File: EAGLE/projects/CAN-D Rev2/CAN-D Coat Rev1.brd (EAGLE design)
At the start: 55.3 x 89.2 mm, 10 parts, among them P1 LCW-106-XX-X-S, P2 LCW-106-XX-X-S, SW1 SCHURTER-LSH-1301.9314, SW2 SCHURTER-LSH-1301.9314, SW3 SCHURTER-LSH-1301.9314

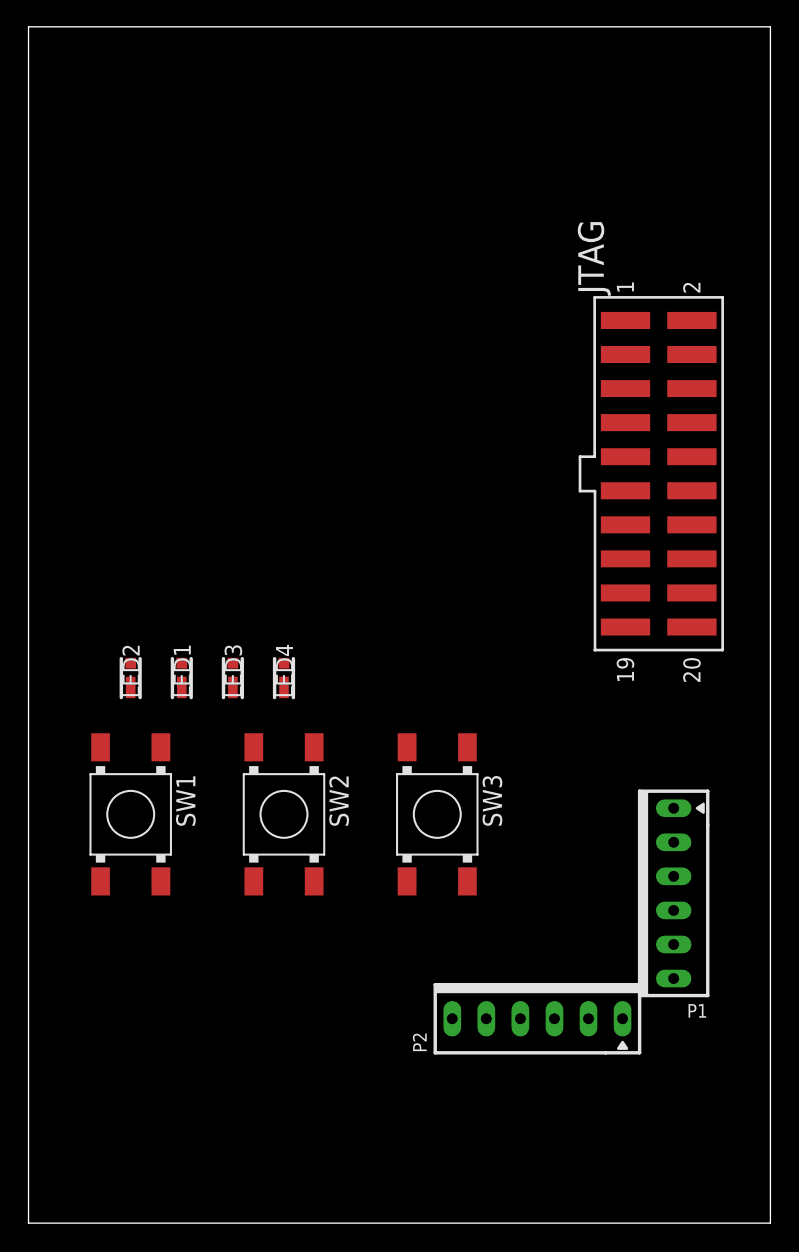
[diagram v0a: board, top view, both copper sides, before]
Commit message: Clean up EAGLE files
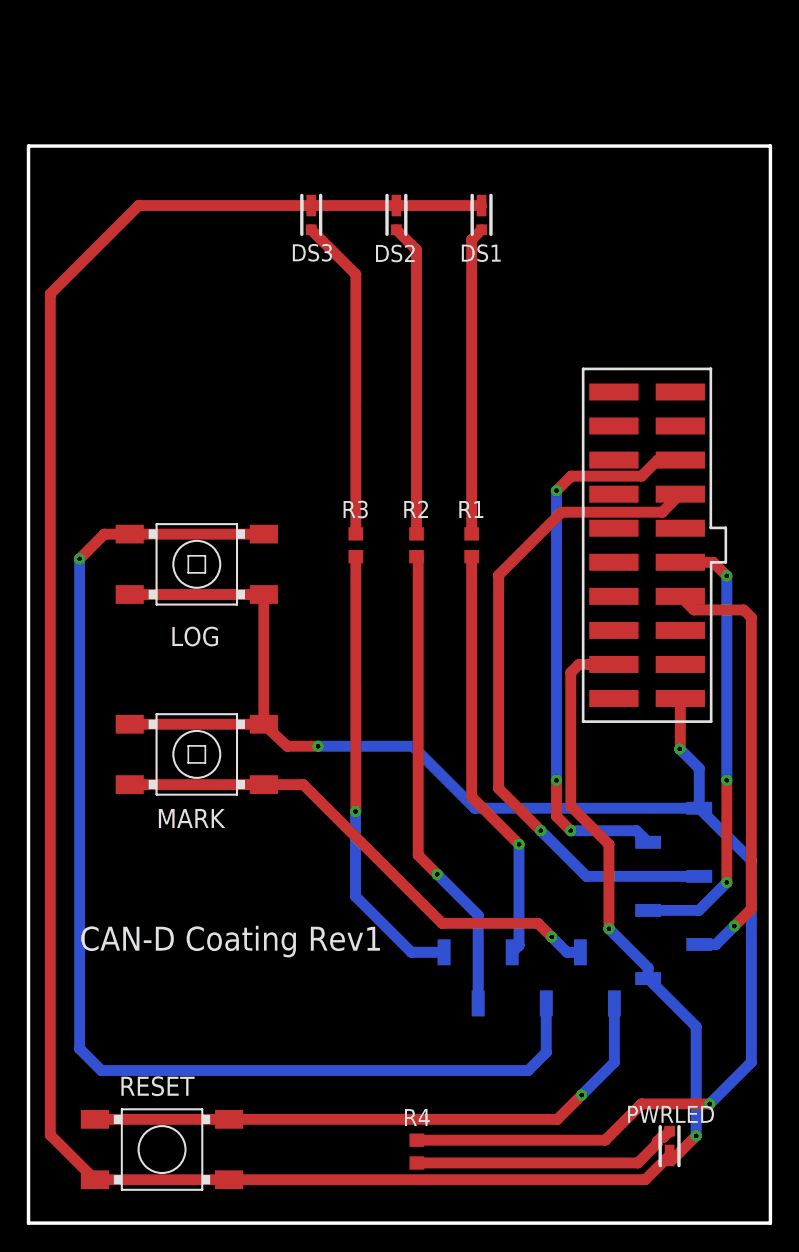
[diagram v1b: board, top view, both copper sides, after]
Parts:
- removed LED1, LED2, LED3, LED4: L130-6580001400001, L130-6580001400001:L130-6580001400001
- removed P1, P2: LCW-106-XX-X-S, con-samtec:LCW-106-XX-X-S
- removed SW1, SW2, SW3: SCHURTER-LSH-1301.9314, schurter_switches_LSH_SMS:LSH
- added DS1, DS2, DS3, PWRLED: LED, CAN-D:L130-6580001400001
- added J1, J2: RECEPTACLE, CAN-D:SSM-106-L-SV-K-TR
- added LOG, MARK: BUTTONSPLUNGER, CAN-D:TL3301SPF260QG
- added R1, R2, R4: 550, CAN-D:R0603
- added R3: 550, rcl:R0603
- added RESET: BUTTONS, CAN-D:1301.9314
- JTAG: value SAMTEC-TSM-110-01-X-DVJ -> JTAG-HEADERJ; device SAMTEC-TSM-110-01-X-DV:SAMTEC-TSM-110-01-X-DV -> CAN-D:TSM-110-02-L-DV-A-P-TR
- moved JTAG 5.40 mm to (46.1, 50.5), turned to 90 degrees
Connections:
- removed net N$1: P1.1
- removed net N$11: P2.5
- removed net N$12: P2.6
- removed net N$2: P1.2
- removed net N$3: P1.3
- removed net N$4: P1.4
- removed net N$5: P1.5
- removed net N$6: P1.6
- new net GND: DS1.2, DS2.2, DS3.2, J1.6, JTAG.4, PWRLED.2, RESET.NO1, RESET.NO2
- new net LED1: J2.3, R1.1
- new net LED2: J2.2, R2.1
- new net LED3: J2.1, R3.1
- new net LOG: J2.4, LOG.C1, LOG.C2
- new net MARK: J2.5, MARK.C1, MARK.C2
- new net NJTRST: J1.2, JTAG.15
- new net RESET: J2.6, RESET.C1, RESET.C2
- new net SWCLK: J1.4, JTAG.9
- new net SWDIO: J1.5, JTAG.7
- new net SWO: J1.3, JTAG.13
- new net VCC: J1.1, JTAG.1, LOG.NO1, LOG.NO2, MARK.NO1, MARK.NO2, R4.1
- net N$10: now also PWRLED.1, R4.2; no longer P2.4
- net N$7: now also DS1.1, R1.2; no longer P2.1
- net N$8: now also DS2.1, R2.2; no longer P2.2
- net N$9: now also DS3.1, R3.2; no longer P2.3
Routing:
- net GND: track 0.00 -> 190.8 mm, vias 0 -> 2
- net VCC: track 0.00 -> 121.4 mm, vias 0 -> 3
- net LOG: track 0.00 -> 90.7 mm, vias 0 -> 1
- net SWO: track 0.00 -> 49.6 mm, vias 0 -> 1
- net RESET: track 0.00 -> 44.9 mm, vias 0 -> 1
- net NJTRST: track 0.00 -> 42.1 mm, vias 0 -> 3
- net MARK: track 0.00 -> 38.8 mm, vias 0 -> 1
- net LED2: track 0.00 -> 35.2 mm, vias 0 -> 1
- net LED3: track 0.00 -> 33.7 mm, vias 0 -> 1
- net SWCLK: track 0.00 -> 33.5 mm, vias 0 -> 3
- net SWDIO: track 0.00 -> 32.7 mm, vias 0 -> 1
- net LED1: track 0.00 -> 31.2 mm, vias 0 -> 1
- net N$9: track 0.00 -> 24.1 mm
- net N$8: track 0.00 -> 23.3 mm
- net N$7: track 0.00 -> 23.0 mm
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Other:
- board size 55.3 x 89.2 mm -> 55.3 x 80.3 mm
- board text added: "CAN-D Coating Rev1"
- board text added: "GND"
- board text added: "NJTRST"
- board text added: "SWCLK"
- board text added: "SWDIO"
- board text added: "SWO"
- board text added: "VTref"
